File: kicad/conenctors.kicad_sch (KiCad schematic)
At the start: 8 parts, among them J3 USB4105-GF-A, J6 Conn_02x12_Counter_Clockwise

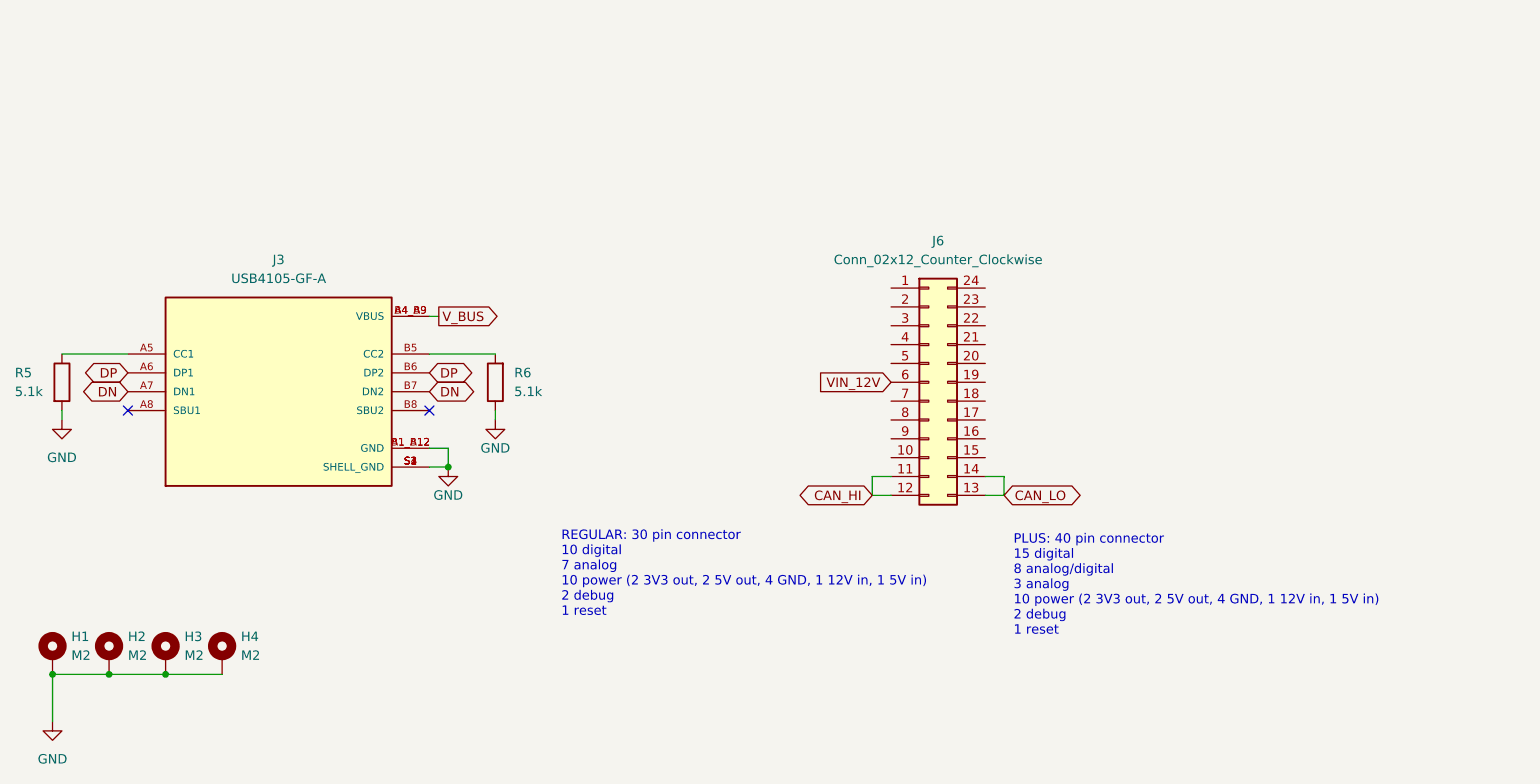
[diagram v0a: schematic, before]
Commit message: Connected all remaining unconnected pins
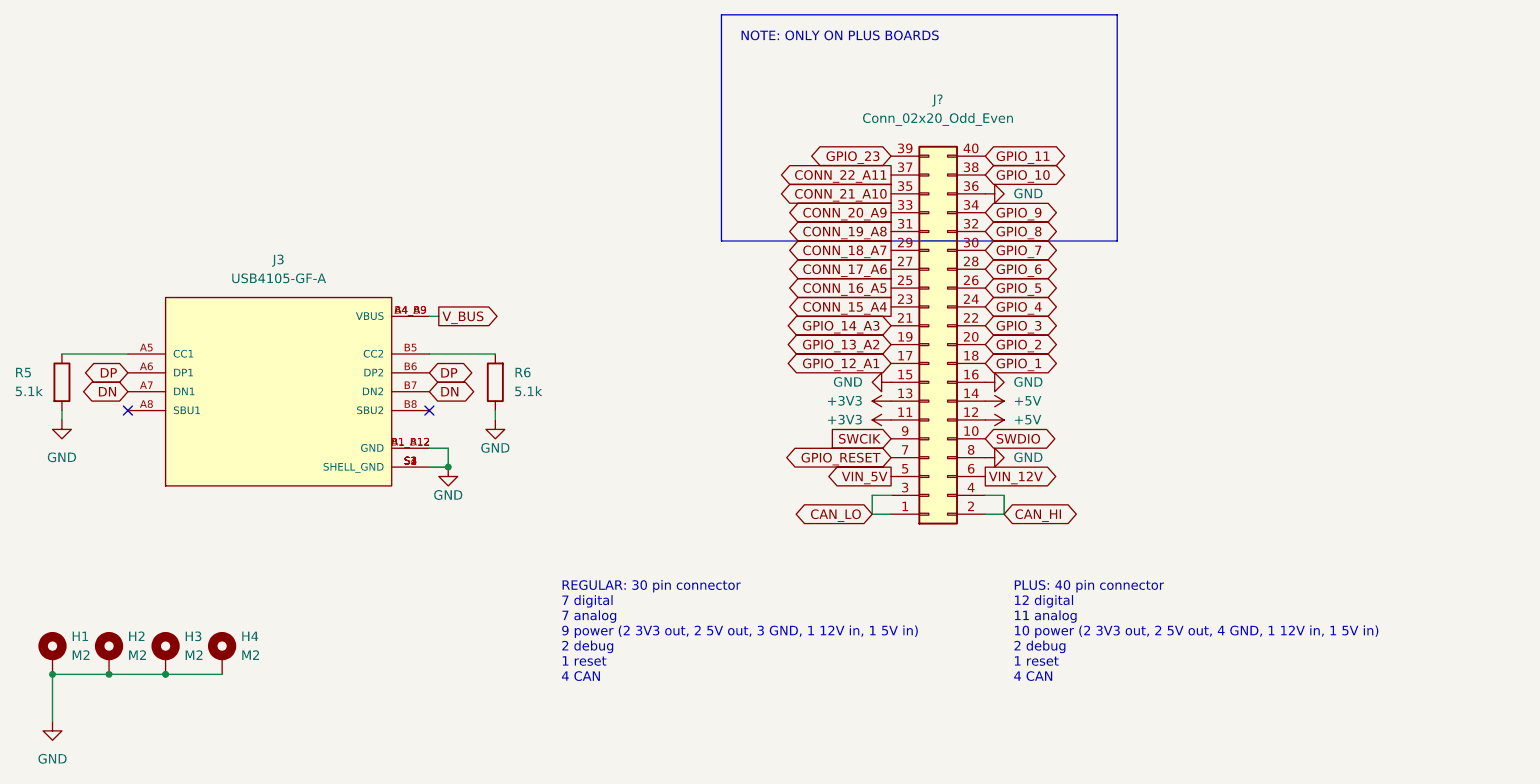
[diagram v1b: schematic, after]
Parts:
- removed J6: Conn_02x12_Counter_Clockwise, Connector_JST:JST_PHD_B24B-PHDSS_2x12_P2.00mm_Vertical, symbol Connector_Generic:Conn_02x12_Counter_Clockwise
- added J?: Conn_02x20_Odd_Even, Connector_JST:JST_PHD_B24B-PHDSS_2x12_P2.00mm_Vertical, symbol Connector_Generic:Conn_02x20_Odd_Even
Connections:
- net CAN_HI: now also J?.2 (Pin_2), J?.4 (Pin_4)
- net CAN_LO: now also J?.1 (Pin_1), J?.3 (Pin_3)
- net GND: now also J?.15 (Pin_15), J?.16 (Pin_16), J?.36 (Pin_36), J?.8 (Pin_8)
- net VIN_12V: now also J?.6 (Pin_6)
- new net +3V3: J?.11 (Pin_11), J?.13 (Pin_13)
- new net +5V: J?.12 (Pin_12), J?.14 (Pin_14)
- new net CONN_15_A4: J?.23 (Pin_23)
- new net CONN_16_A5: J?.25 (Pin_25)
- new net CONN_17_A6: J?.27 (Pin_27)
- new net CONN_18_A7: J?.29 (Pin_29)
- new net CONN_19_A8: J?.31 (Pin_31)
- new net CONN_20_A9: J?.33 (Pin_33)
- new net CONN_21_A10: J?.35 (Pin_35)
- new net CONN_22_A11: J?.37 (Pin_37)
- new net GPIO_1: J?.18 (Pin_18)
- new net GPIO_10: J?.38 (Pin_38)
- new net GPIO_11: J?.40 (Pin_40)
- new net GPIO_12_A1: J?.17 (Pin_17)
- new net GPIO_13_A2: J?.19 (Pin_19)
- new net GPIO_14_A3: J?.21 (Pin_21)
- new net GPIO_2: J?.20 (Pin_20)
- new net GPIO_23: J?.39 (Pin_39)
- new net GPIO_3: J?.22 (Pin_22)
- new net GPIO_4: J?.24 (Pin_24)
- new net GPIO_5: J?.26 (Pin_26)
- new net GPIO_6: J?.28 (Pin_28)
- new net GPIO_7: J?.30 (Pin_30)
- new net GPIO_8: J?.32 (Pin_32)
- new net GPIO_9: J?.34 (Pin_34)
- new net GPIO_RESET: J?.7 (Pin_7)
- new net SWCIK: J?.9 (Pin_9)
- new net SWDIO: J?.10 (Pin_10)
- new net VIN_5V: J?.5 (Pin_5)
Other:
- note added: "NOTE: ONLY ON PLUS BOARDS"
- note added: "PLUS: 40 pin connector 12 digital 11 analog 10 power (2 3V3 out, 2 5V out, 4 GND, 1 12V in, 1 5V in) 2 debug 1 reset 4 CAN"
- note added: "REGULAR: 30 pin connector 7 digital 7 analog 9 power (2 3V3 out, 2 5V out, 3 GND, 1 12V in, 1 5V in) 2 debug 1 reset 4 CAN"
- note removed: "PLUS: 40 pin connector 15 digital 8 analog/digital 3 analog 10 power (2 3V3 out, 2 5V out, 4 GND, 1 12V in, 1 5V in) 2 debug 1 reset"
- note removed: "REGULAR: 30 pin connector 10 digital 7 analog 10 power (2 3V3 out, 2 5V out, 4 GND, 1 12V in, 1 5V in) 2 debug 1 reset"
